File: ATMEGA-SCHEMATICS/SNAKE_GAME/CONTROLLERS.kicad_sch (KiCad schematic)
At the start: 20 parts, among them J1 UART_ESP, J12 USB_ASP, J13 UART_TERM, J14 BUTTONS, J17 JOYSTICK

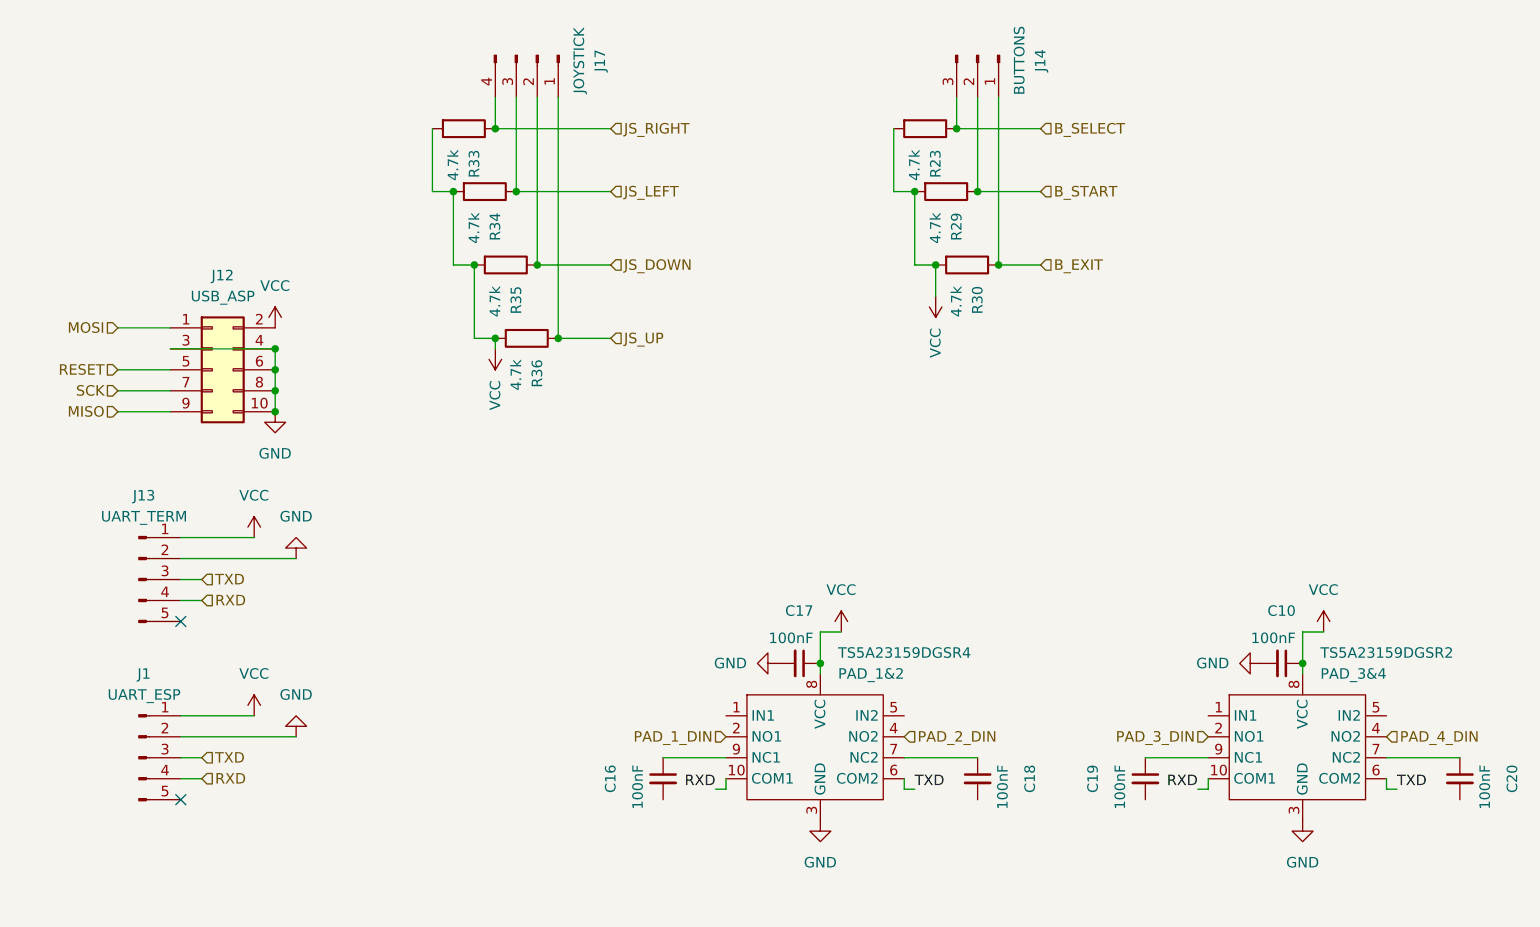
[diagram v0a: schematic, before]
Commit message: .
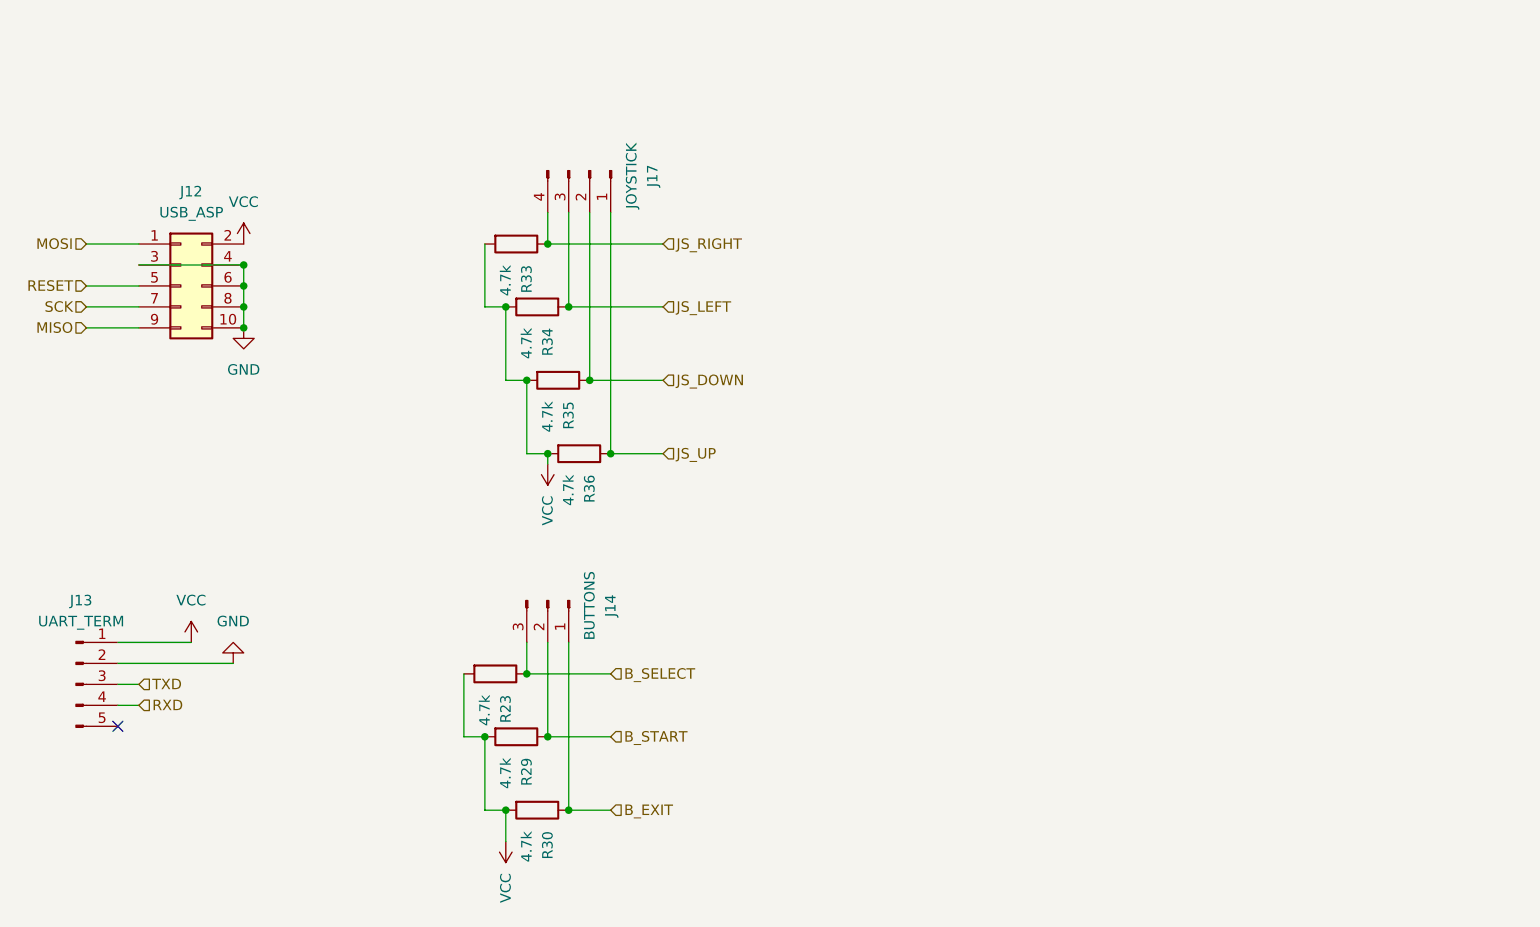
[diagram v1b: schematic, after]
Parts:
- removed C10, C16, C17, C18, C19, C20: 100nF, Capacitor_THT:C_Disc_D7.5mm_W5.0mm_P5.00mm, symbol Device:C_Small
- removed J1: UART_ESP, Connector_PinSocket_2.54mm:PinSocket_1x04_P2.54mm_Vertical, symbol Connector:Conn_01x05_Pin
- removed TS5A23159DGSR2: PAD_3&4, symbol Lucas_Lib:TS5A23159DGSR
- removed TS5A23159DGSR4: PAD_1&2, symbol Lucas_Lib:TS5A23159DGSR
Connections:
- no-connect marks 2 -> 1
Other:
- moved on the sheet: J12, J13, J14, J17, R23, R29, R30, R33, R34, R35, R36

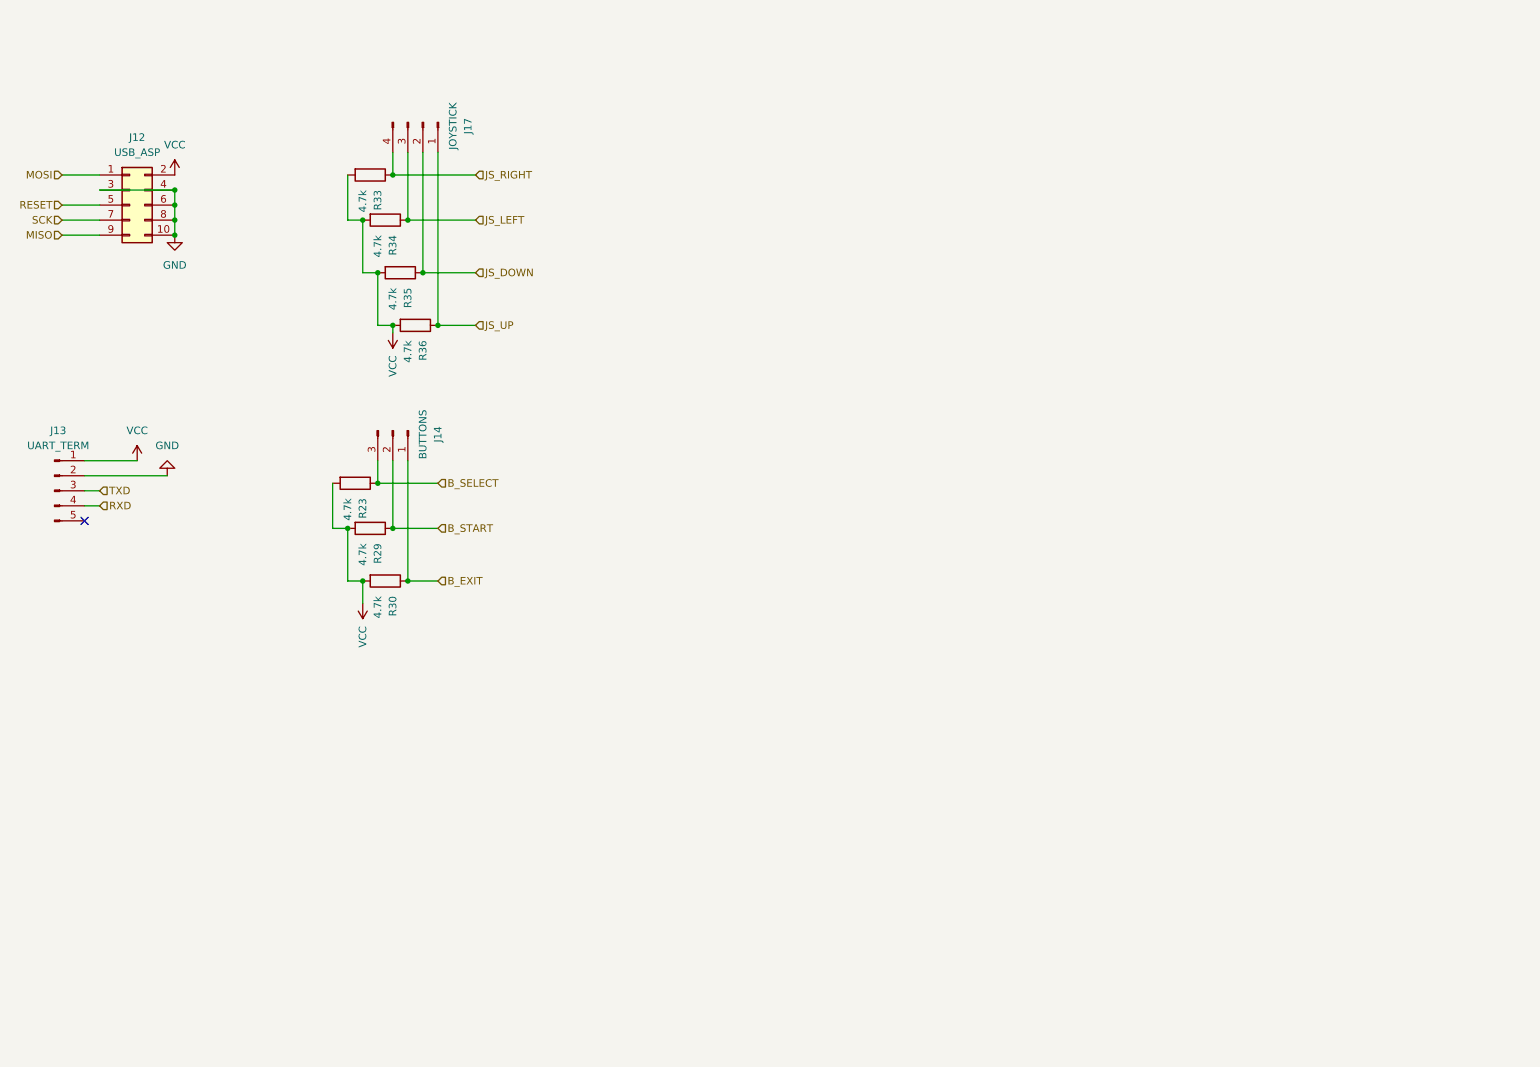
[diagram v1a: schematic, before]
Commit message: .
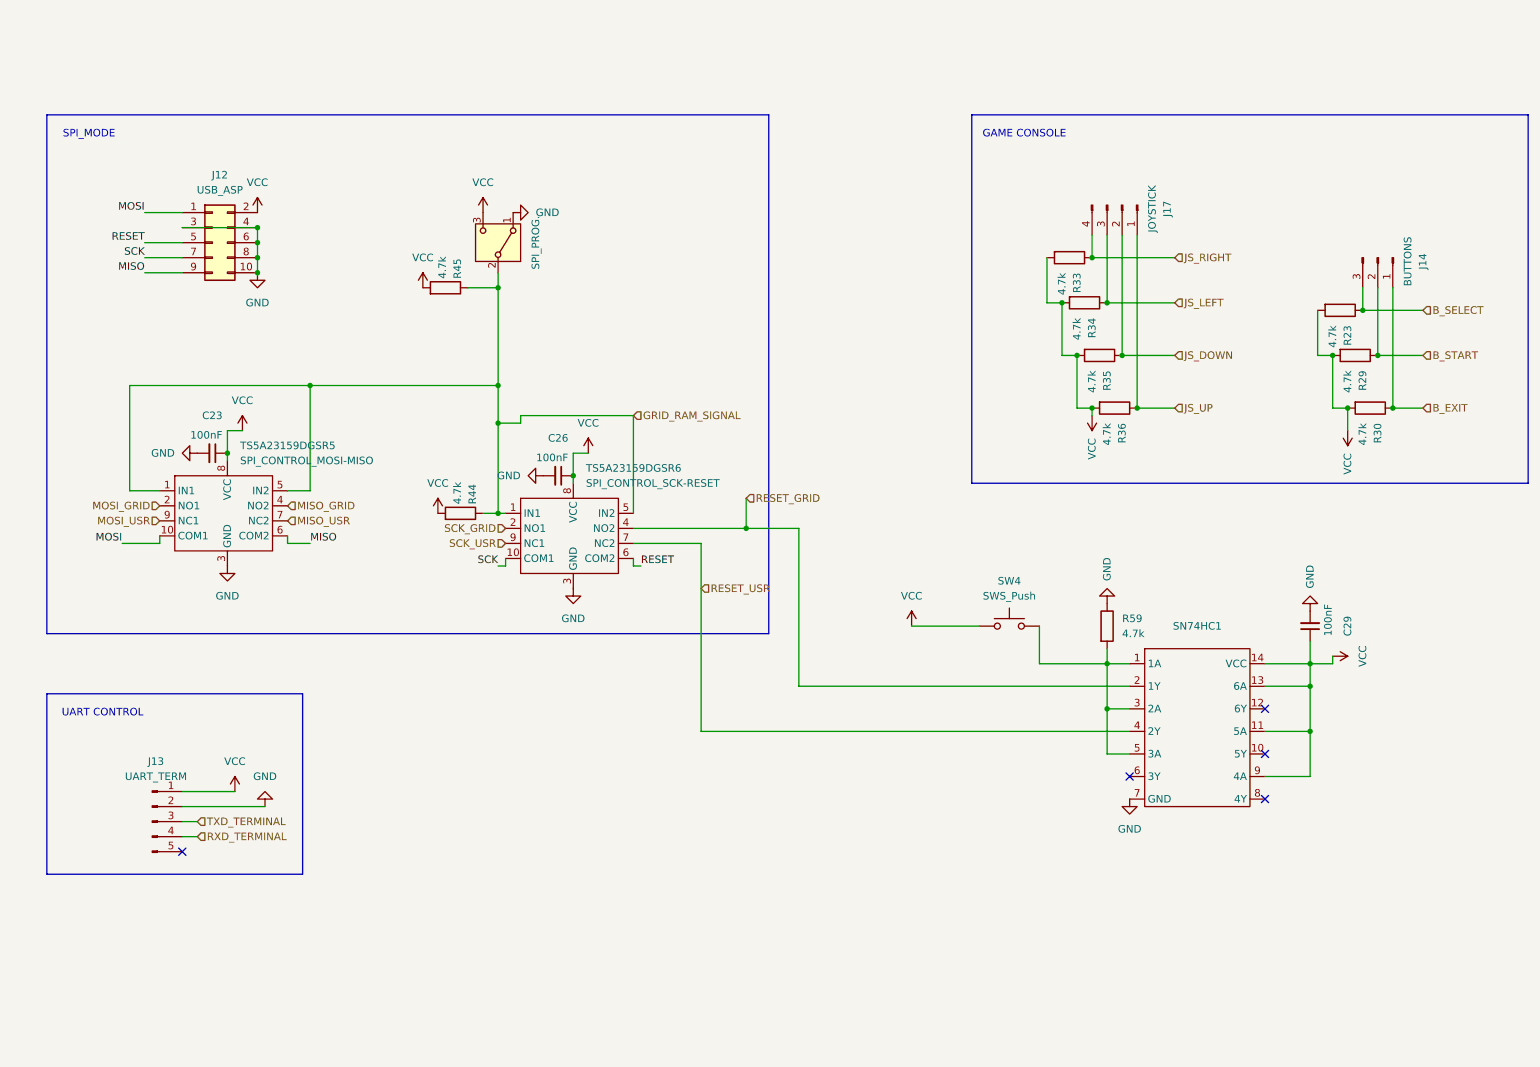
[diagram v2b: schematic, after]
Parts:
- added C23, C26, C29: 100nF, Capacitor_THT:C_Disc_D7.5mm_W5.0mm_P5.00mm, symbol Device:C_Small
- added R44, R45, R59: 4.7k, Resistor_THT:R_Axial_DIN0207_L6.3mm_D2.5mm_P10.16mm_Horizontal, symbol Device:R
- added SN74HC1: ~, Package_DIP:CERDIP-14_W7.62mm_SideBrazed_Socket, symbol lucasLib:SN74HC14N
- added SW4: SWS_Push, Button_Switch_THT:SW_PUSH_6mm, symbol Switch:SW_Push
- added SW6: SPI_PROG., Button_Switch_THT:SW_Slide_SPDT_Straight_CK_OS102011MS2Q, symbol Switch:SW_SPDT
- added TS5A23159DGSR5: SPI_CONTROL_MOSI-MISO, LucasLib:TS5A23159DGSR, symbol Lucas_Lib:TS5A23159DGSR
- added TS5A23159DGSR6: SPI_CONTROL_SCK-RESET, LucasLib:TS5A23159DGSR, symbol Lucas_Lib:TS5A23159DGSR
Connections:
- net GND: now also C23.2, C26.2, C29.2, R59.1, SN74HC1.7 (GND), SW6.1 (A), TS5A23159DGSR5.3 (GND), TS5A23159DGSR6.3 (GND)
- net MISO: now also TS5A23159DGSR5.6 (COM2)
- net MOSI: now also TS5A23159DGSR5.10 (COM1)
- net RESET: now also TS5A23159DGSR6.6 (COM2)
- net SCK: now also TS5A23159DGSR6.10 (COM1)
- net VCC: now also C23.1, C26.1, C29.1, R44.2, R45.2, SN74HC1.11 (5A), SN74HC1.13 (6A), SN74HC1.14 (VCC), SN74HC1.9 (4A), SW4.2, SW6.3 (C), TS5A23159DGSR5.8 (VCC), TS5A23159DGSR6.8 (VCC)
- net RXD renamed RXD_TERMINAL
- net TXD renamed TXD_TERMINAL
- new net: R59.2, SN74HC1.1 (1A), SN74HC1.3 (2A), SN74HC1.5 (3A), SW4.1
- new net GRID_RAM_SIGNAL: R44.1, R45.1, SW6.2 (B), TS5A23159DGSR5.1 (IN1), TS5A23159DGSR5.5 (IN2), TS5A23159DGSR6.1 (IN1), TS5A23159DGSR6.5 (IN2)
- new net MISO_GRID: TS5A23159DGSR5.4 (NO2)
- new net MISO_USR: TS5A23159DGSR5.7 (NC2)
- new net MOSI_GRID: TS5A23159DGSR5.2 (NO1)
- new net MOSI_USR: TS5A23159DGSR5.9 (NC1)
- new net RESET_GRID: SN74HC1.2 (1Y), TS5A23159DGSR6.4 (NO2)
- new net RESET_USR: SN74HC1.4 (2Y), TS5A23159DGSR6.7 (NC2)
- new net SCK_GRID: TS5A23159DGSR6.2 (NO1)
- new net SCK_USR: TS5A23159DGSR6.9 (NC1)
- no-connect marks 1 -> 5
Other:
- note added: "GAME CONSOLE"
- note added: "SPI_MODE"
- note added: "UART CONTROL"
- moved on the sheet: J12, J13, J14, J17, R23, R29, R30, R33, R34, R35, R36

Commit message: ..
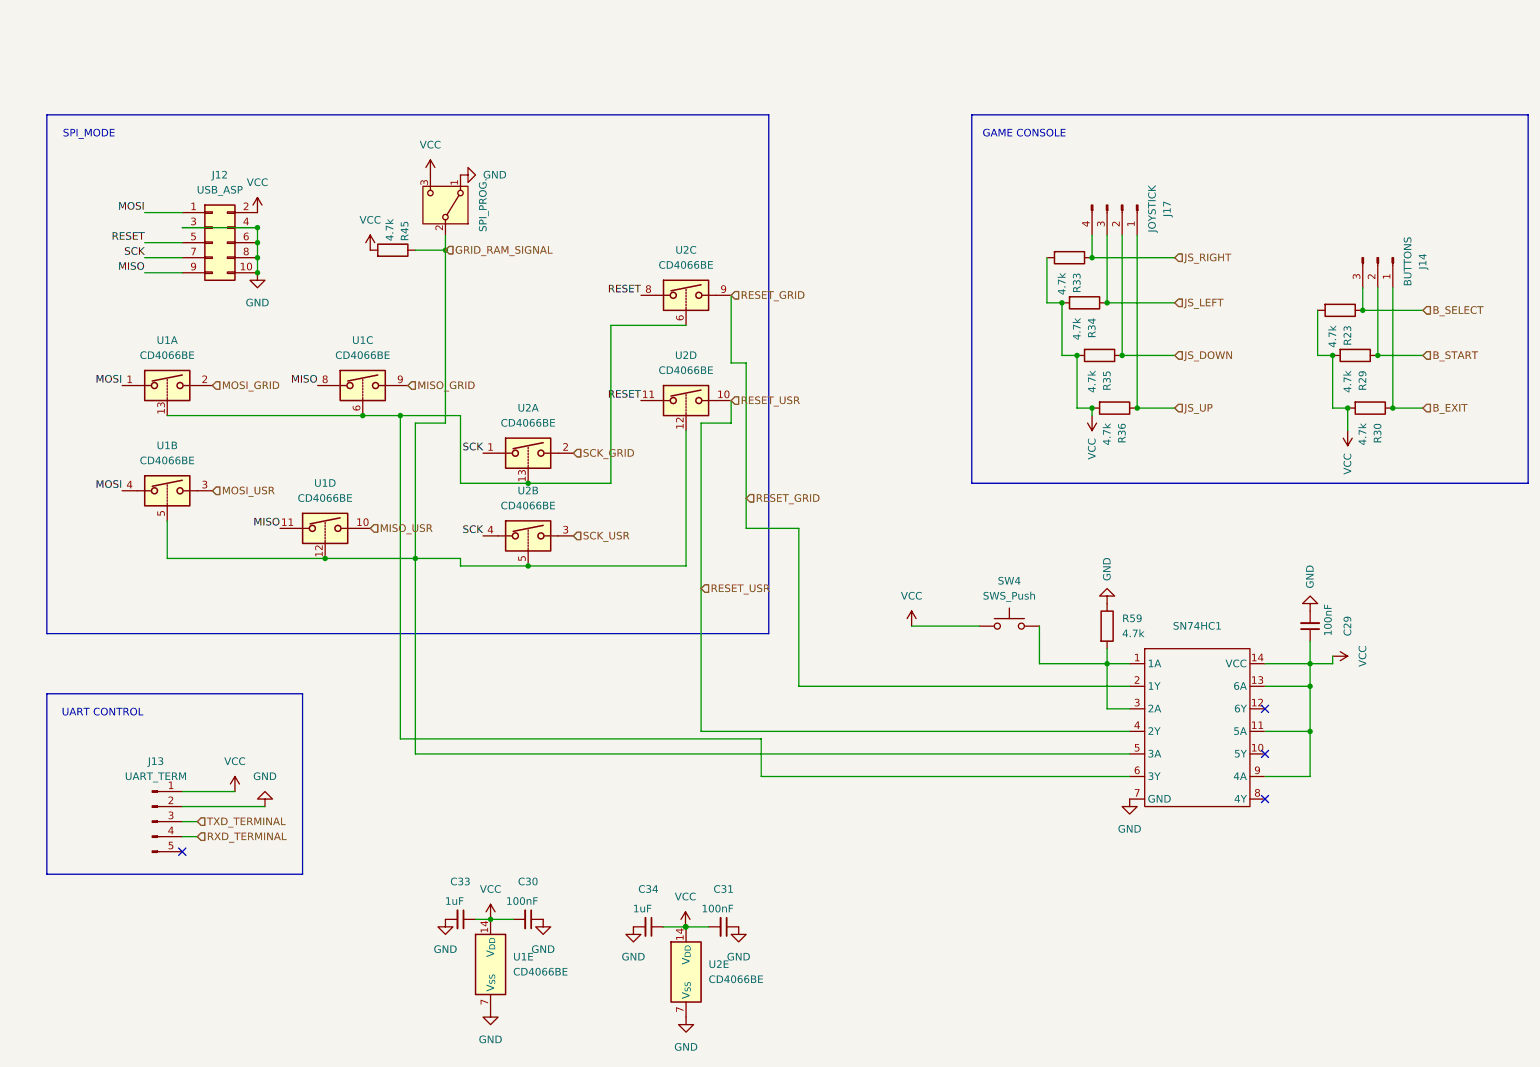
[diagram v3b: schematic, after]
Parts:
- removed C23, C26: 100nF, Capacitor_THT:C_Disc_D7.5mm_W5.0mm_P5.00mm, symbol Device:C_Small
- removed R44: 4.7k, Resistor_THT:R_Axial_DIN0207_L6.3mm_D2.5mm_P10.16mm_Horizontal, symbol Device:R
- removed TS5A23159DGSR5: SPI_CONTROL_MOSI-MISO, LucasLib:TS5A23159DGSR, symbol Lucas_Lib:TS5A23159DGSR
- removed TS5A23159DGSR6: SPI_CONTROL_SCK-RESET, LucasLib:TS5A23159DGSR, symbol Lucas_Lib:TS5A23159DGSR
- added C30, C31: 100nF, Capacitor_THT:C_Disc_D7.5mm_W5.0mm_P5.00mm, symbol Device:C_Small
- added C33, C34: 1uF, Capacitor_THT:C_Disc_D7.5mm_W5.0mm_P5.00mm, symbol Device:C_Small
- added U1, U2: CD4066BE, Package_DIP:DIP-14_W7.62mm, symbol Analog_Switch:CD4066BE
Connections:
- net GND: now also C30.1, C31.1, C33.2, C34.2, U1.7 (V_{SS}), U2.7 (V_{SS})
- net GRID_RAM_SIGNAL: now also SN74HC1.5 (3A), U1.12, U1.5, U2.12, U2.5
- net MISO: now also U1.11, U1.8
- net MISO_GRID: now also U1.9
- net MISO_USR: now also U1.10
- net MOSI: now also U1.1, U1.4
- net MOSI_GRID: now also U1.2
- net MOSI_USR: now also U1.3
- net RESET: now also U2.11, U2.8
- net RESET_GRID: now also U2.9
- net RESET_USR: now also U2.10
- net SCK: now also U2.1, U2.4
- net SCK_GRID: now also U2.2
- net SCK_USR: now also U2.3
- net VCC: now also C30.2, C31.2, C33.1, C34.1, U1.14 (V_{DD}), U2.14 (V_{DD})
- net at R59.2, SN74HC1.1 (1A), SN74HC1.3 (2A)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: no longer SN74HC1.5 (3A)
- net at SN74HC1.6 (3Y): now also U1.13, U1.6, U2.13, U2.6
- no-connect marks 5 -> 4
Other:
- moved on the sheet: R45
